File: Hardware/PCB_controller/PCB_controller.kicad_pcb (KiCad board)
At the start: 4 copper layers, 46.5 x 59 mm, 72 parts, among them J1 Conn_01x02, J2 Conn_01x06, J3 Conn_01x04, J4 Conn_ST_STDC14, SW1 SW_SPST, SW10 SW_SPST, SW11 SW_SPST, SW2 SW_SPST, SW3 SW_SPST, SW4 SW_SPST, SW5 SW_SPST, SW6 SW_SPST, SW7 SW_SPST, SW8 SW_SPST, SW9 SW_SPST, U1 STM32G431KBTx, U2 AZ1117-3.3

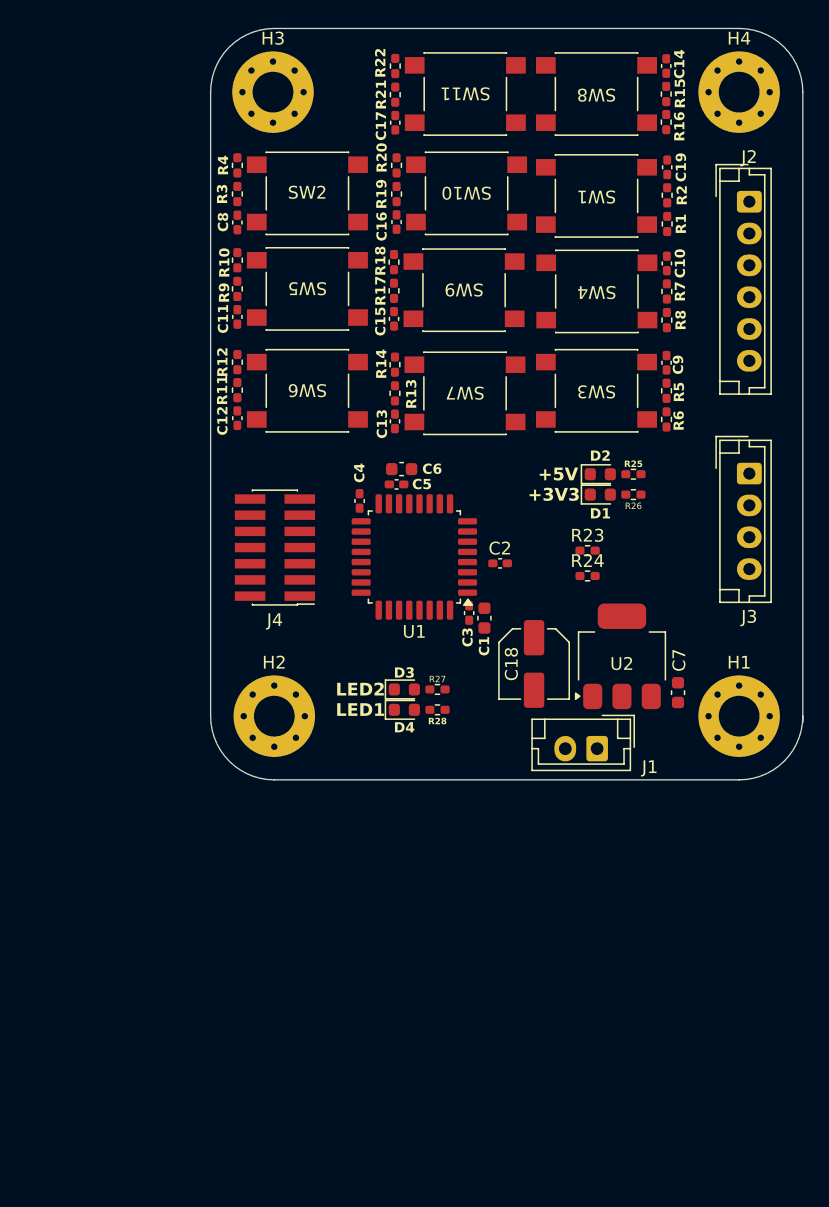
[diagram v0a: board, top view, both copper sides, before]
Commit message: finished controller PCB
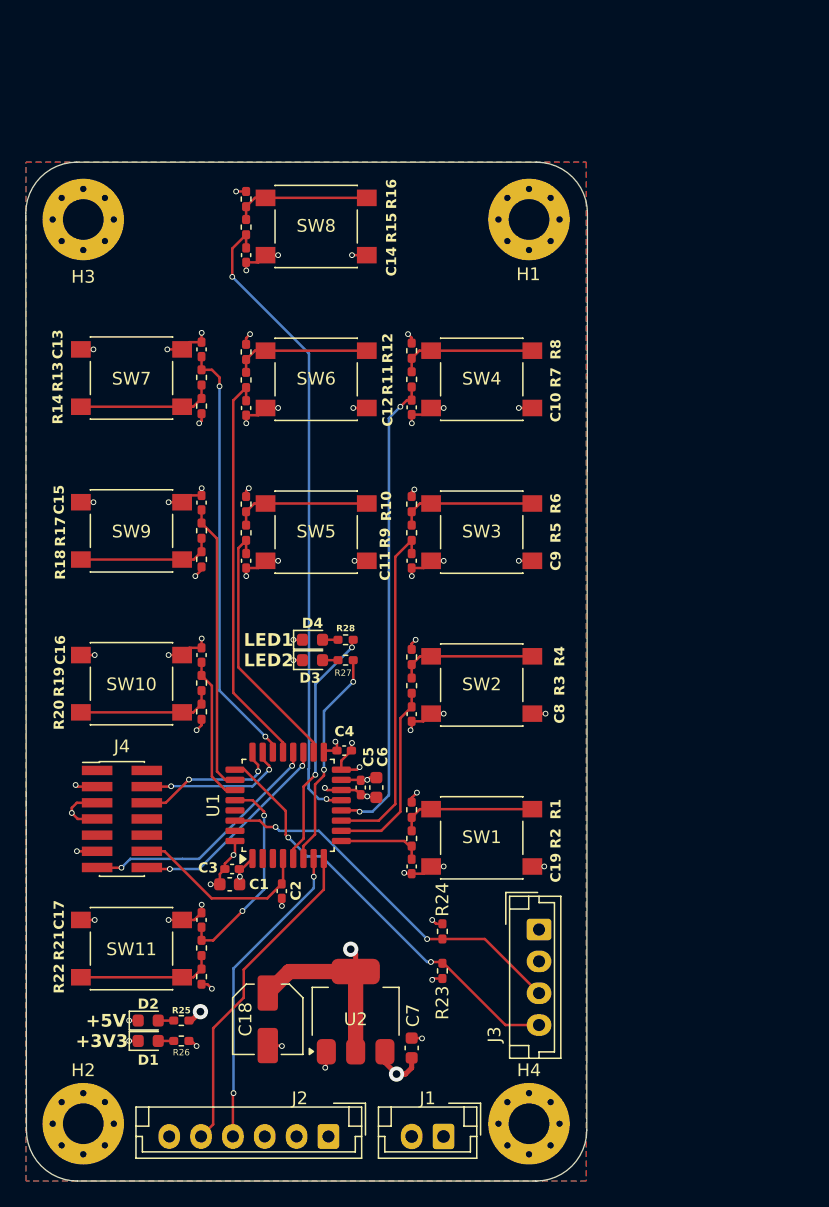
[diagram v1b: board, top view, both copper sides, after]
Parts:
- moved H4 82.7 mm to (162.0, 130.0)
- moved J2 80.5 mm to (146.2, 131.0), turned to 180 degrees
- moved R22 73.1 mm to (136.3, 118.5), turned to 90 degrees
- moved SW11 72.1 mm to (130.8, 116.3), turned to 180 degrees
- moved R21 68.7 mm to (136.3, 116.2), turned to -90 degrees
- moved C17 64.4 mm to (136.3, 114.0), turned to 90 degrees
- moved C19 58.5 mm to (152.8, 109.8), turned to -90 degrees
- moved D1 55.7 mm to (132.1, 123.5)
- moved D2 55.7 mm to (132.1, 121.9)
- moved R25 55.7 mm to (134.7, 121.9)
- moved R26 55.7 mm to (134.7, 123.5)
- moved R2 54.3 mm to (152.8, 107.6), turned to 90 degrees
- moved SW1 51.1 mm to (158.3, 107.5), turned to 0 degrees
- moved R1 50.2 mm to (152.8, 105.3), turned to -90 degrees
- moved SW10 46.7 mm to (130.8, 95.5), turned to 180 degrees
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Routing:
- net GND: track 0.00 -> 80.2 mm, vias 0 -> 49
- net BTN_8: track 0.00 -> 50.4 mm, vias 0 -> 2
- net BTN_4: track 0.00 -> 37.3 mm, vias 0 -> 2
- net +3.3V: track 0.00 -> 36.8 mm, vias 0 -> 19
- net BTN_7: track 0.00 -> 33.9 mm, vias 0 -> 2
- net I2C1_SCL: track 0.00 -> 33.3 mm, vias 0 -> 2
- net BTN_6: track 0.00 -> 31.7 mm
- net I2C1_SDA: track 0.00 -> 29.5 mm, vias 0 -> 2
- net BTN_3: track 0.00 -> 27.0 mm
- net UART2_HC05_RX: track 0.00 -> 25.8 mm
- net UART2_HC05_TX: track 0.00 -> 24.5 mm, vias 0 -> 2
- net BTN_9: track 0.00 -> 22.7 mm
- net BTN_5: track 0.00 -> 20.4 mm
- net UART1_DEBUG_RX: track 0.00 -> 19.7 mm, vias 0 -> 2
- net LED1: track 0.00 -> 19.1 mm, vias 0 -> 2
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- added copper zone on In1.Cu, net +3.3V
- added copper zone on In1.Cu, net +5V
- added copper zone on B.Cu, net GND
- added copper zone on F.Cu, net GND
- added copper zone on In2.Cu, net GND
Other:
- board size 46.5 x 59 mm -> 44.1 x 80 mm
